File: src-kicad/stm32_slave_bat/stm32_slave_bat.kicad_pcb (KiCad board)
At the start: 2 copper layers, 40 x 50 mm, 26 parts, among them J1 Conn_01x02_Male, J2 Conn_01x02_Male, J3 Conn_02x04_Odd_Even, J4 Conn_01x04_Female, Q1 Si2371EDS, SW1 SW_Push, SW2 SW_DIP_x01, U1 STM32F031F6Px, Y1 8M

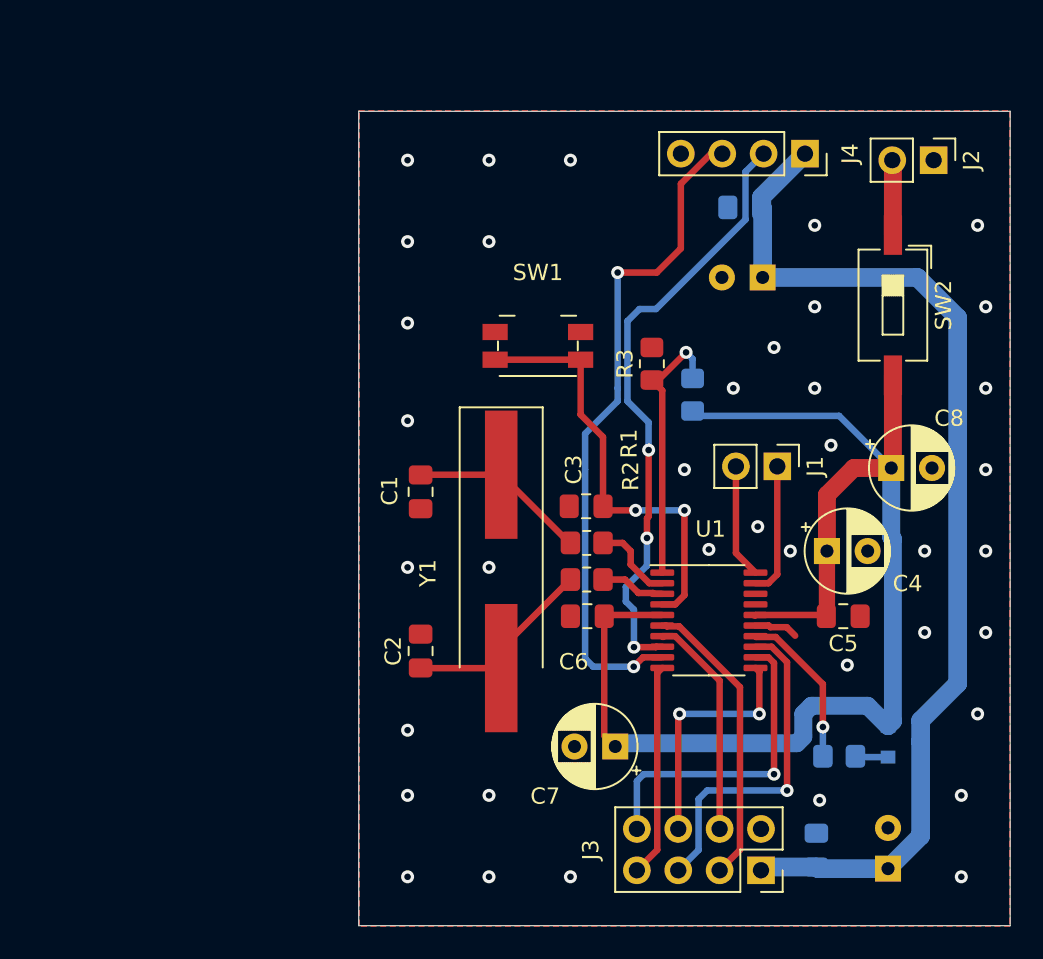
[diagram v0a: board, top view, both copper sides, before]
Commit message: Minor fixes in kicad
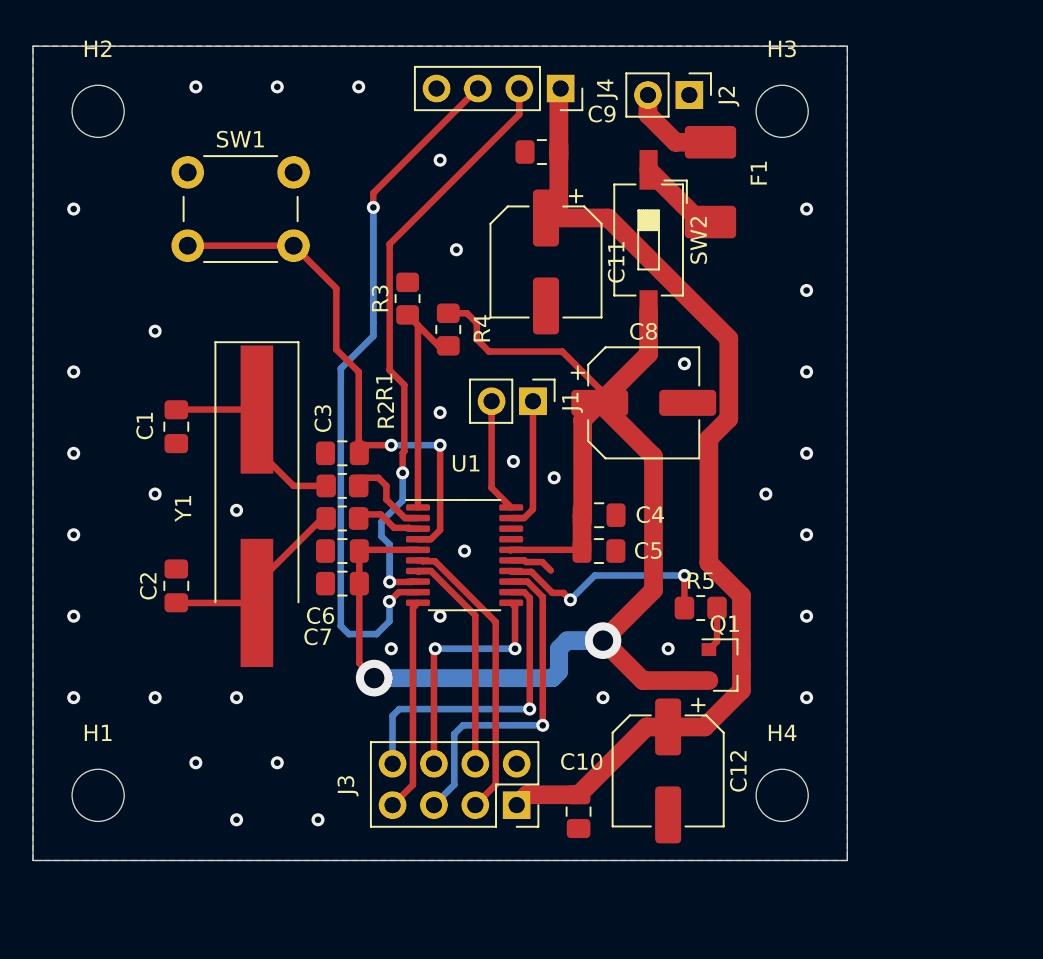
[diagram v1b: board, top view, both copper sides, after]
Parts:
- added F1: Fuse, smd-2410:smd-2410, F.Cu at (241.6, 110.8)
- added H1: MountingHole_Pad, MountingHole:MountingHole_3.2mm_M3_DIN965, F.Cu at (204.0, 146.0)
- added H2: MountingHole_Pad, MountingHole:MountingHole_3.2mm_M3_DIN965, F.Cu at (204.0, 104.0)
- added H3: MountingHole_Pad, MountingHole:MountingHole_3.2mm_M3_DIN965, F.Cu at (246.0, 104.0)
- added H4: MountingHole_Pad, MountingHole:MountingHole_3.2mm_M3_DIN965, F.Cu at (246.0, 146.0)
- C10, C9, Q1, R4, R5: moved to F.Cu
- C11, C12: footprint Capacitor_THT:CP_Radial_D5.0mm_P2.50mm -> Capacitor_SMD:CP_Elec_6.3x5.8; moved to F.Cu
- C4, C7: footprint Capacitor_THT:CP_Radial_D5.0mm_P2.50mm -> Capacitor_SMD:C_0805_2012Metric_Pad1.18x1.45mm_HandSolder
- C8: footprint Capacitor_THT:CP_Radial_D5.0mm_P2.50mm -> Capacitor_SMD:CP_Elec_6.3x5.8
- SW1: footprint Button_Switch_SMD:Panasonic_EVQPUJ_EVQPUA -> Button_Switch_THT:SW_PUSH_6mm_H5mm
- moved SW1 24.0 mm to (209.5, 107.8)
- moved C7 19.5 mm to (219.0, 133.0)
- moved C8 15.7 mm to (237.5, 121.9)
- moved C6 15.6 mm to (219.0, 131.0)
- moved C1 15.5 mm to (208.8, 123.4)
- moved C2 15.5 mm to (208.8, 133.1)
- moved C5 15.5 mm to (234.8, 131.0)
- moved J1 15.5 mm to (230.7, 121.8)
- moved J2 15.5 mm to (240.3, 103.0)
- moved J3 15.5 mm to (229.7, 146.6)
- moved J4 15.5 mm to (232.4, 102.6)
- moved R3 15.5 mm to (223.0, 115.5)
- moved R4 15.5 mm to (225.5, 117.4), turned to 90 degrees
- moved SW2 15.5 mm to (237.8, 111.9)
- moved U1 15.5 mm to (226.5, 131.2)
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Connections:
- C4 pad 1: +3V3 -> GND
- C4 pad 2: GND -> +3V3
- J2 pad 2: Net-(J2-Pad2) -> Net-(F1-Pad1)
- SW2 pad 1: Net-(J2-Pad2) -> Net-(F1-Pad2)
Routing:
- net Net-(F1-Pad1): track 0.00 -> 5.75 mm
- net Net-(C3-Pad2): track 26.7 -> 32.1 mm
- net Net-(F1-Pad2): track 0.00 -> 5.13 mm
- net Net-(J2-Pad2): track 4.67 -> 0.00 mm
- net Net-(R5-Pad1): track 9.79 -> 14.0 mm, vias 1 -> 2
- net Vcc: track 65.2 -> 62.0 mm
- net +3V3: track 83.0 -> 86.0 mm, vias 0 -> 2
- net UART1_RXD: track 41.5 -> 43.9 mm
- net Net-(R3-Pad1): track 16.7 -> 14.9 mm, vias 1 -> 0
- net Net-(C1-Pad1): track 10.9 -> 12.6 mm
- net UART1_TXD: track 37.4 -> 36.5 mm, vias 3 -> 2
- net Net-(Q1-Pad1): track 2.02 -> 2.76 mm
- net GND: vias 38 -> 37
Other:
- board size 40 x 50 mm -> 50 x 50 mm
